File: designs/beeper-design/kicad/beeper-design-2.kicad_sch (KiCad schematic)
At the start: 26 parts, among them U14 EVPBB4A9B000, U15 EVPBB4A9B000, U16 EVPBB4A9B000, U4 DA7212-01UM2, U9 LSM6DSOXTR

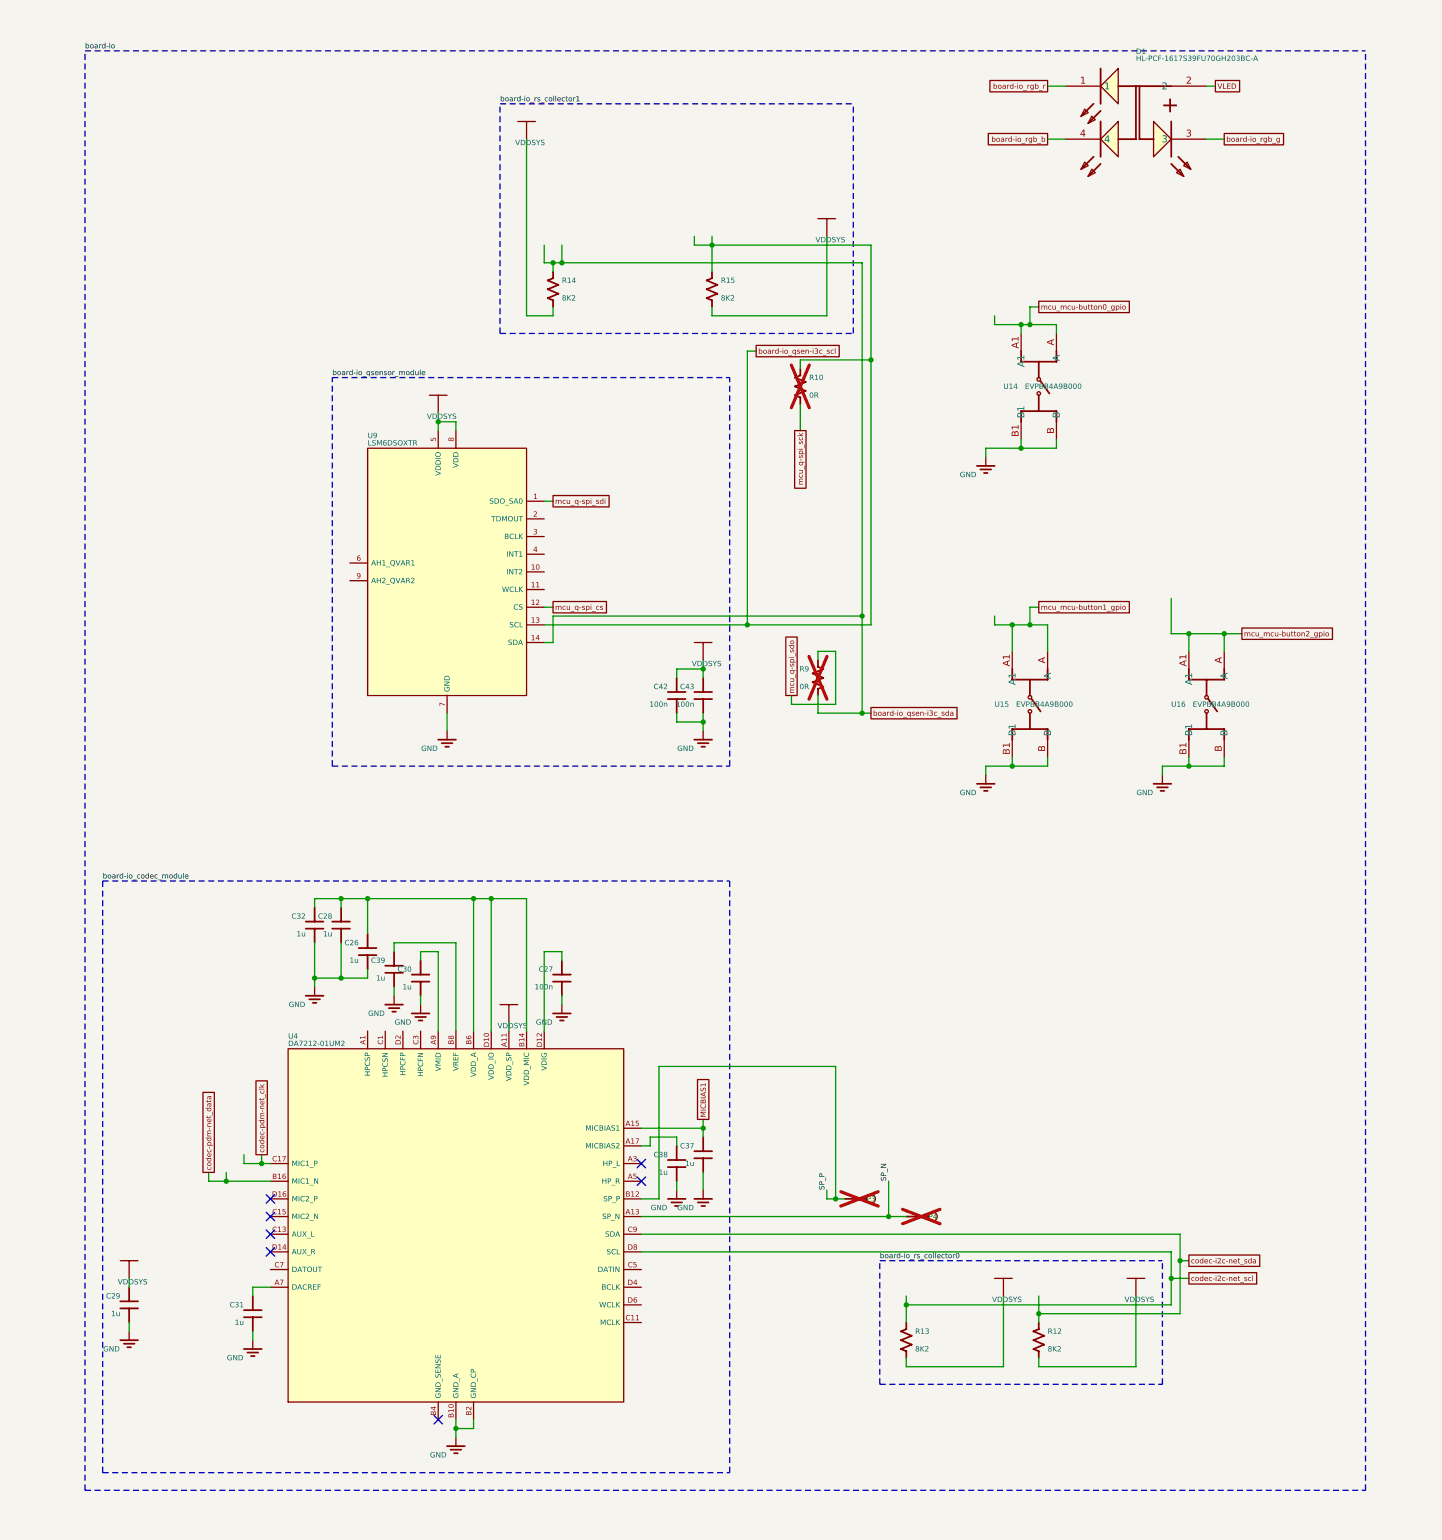
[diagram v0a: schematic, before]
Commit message: kicad exported data
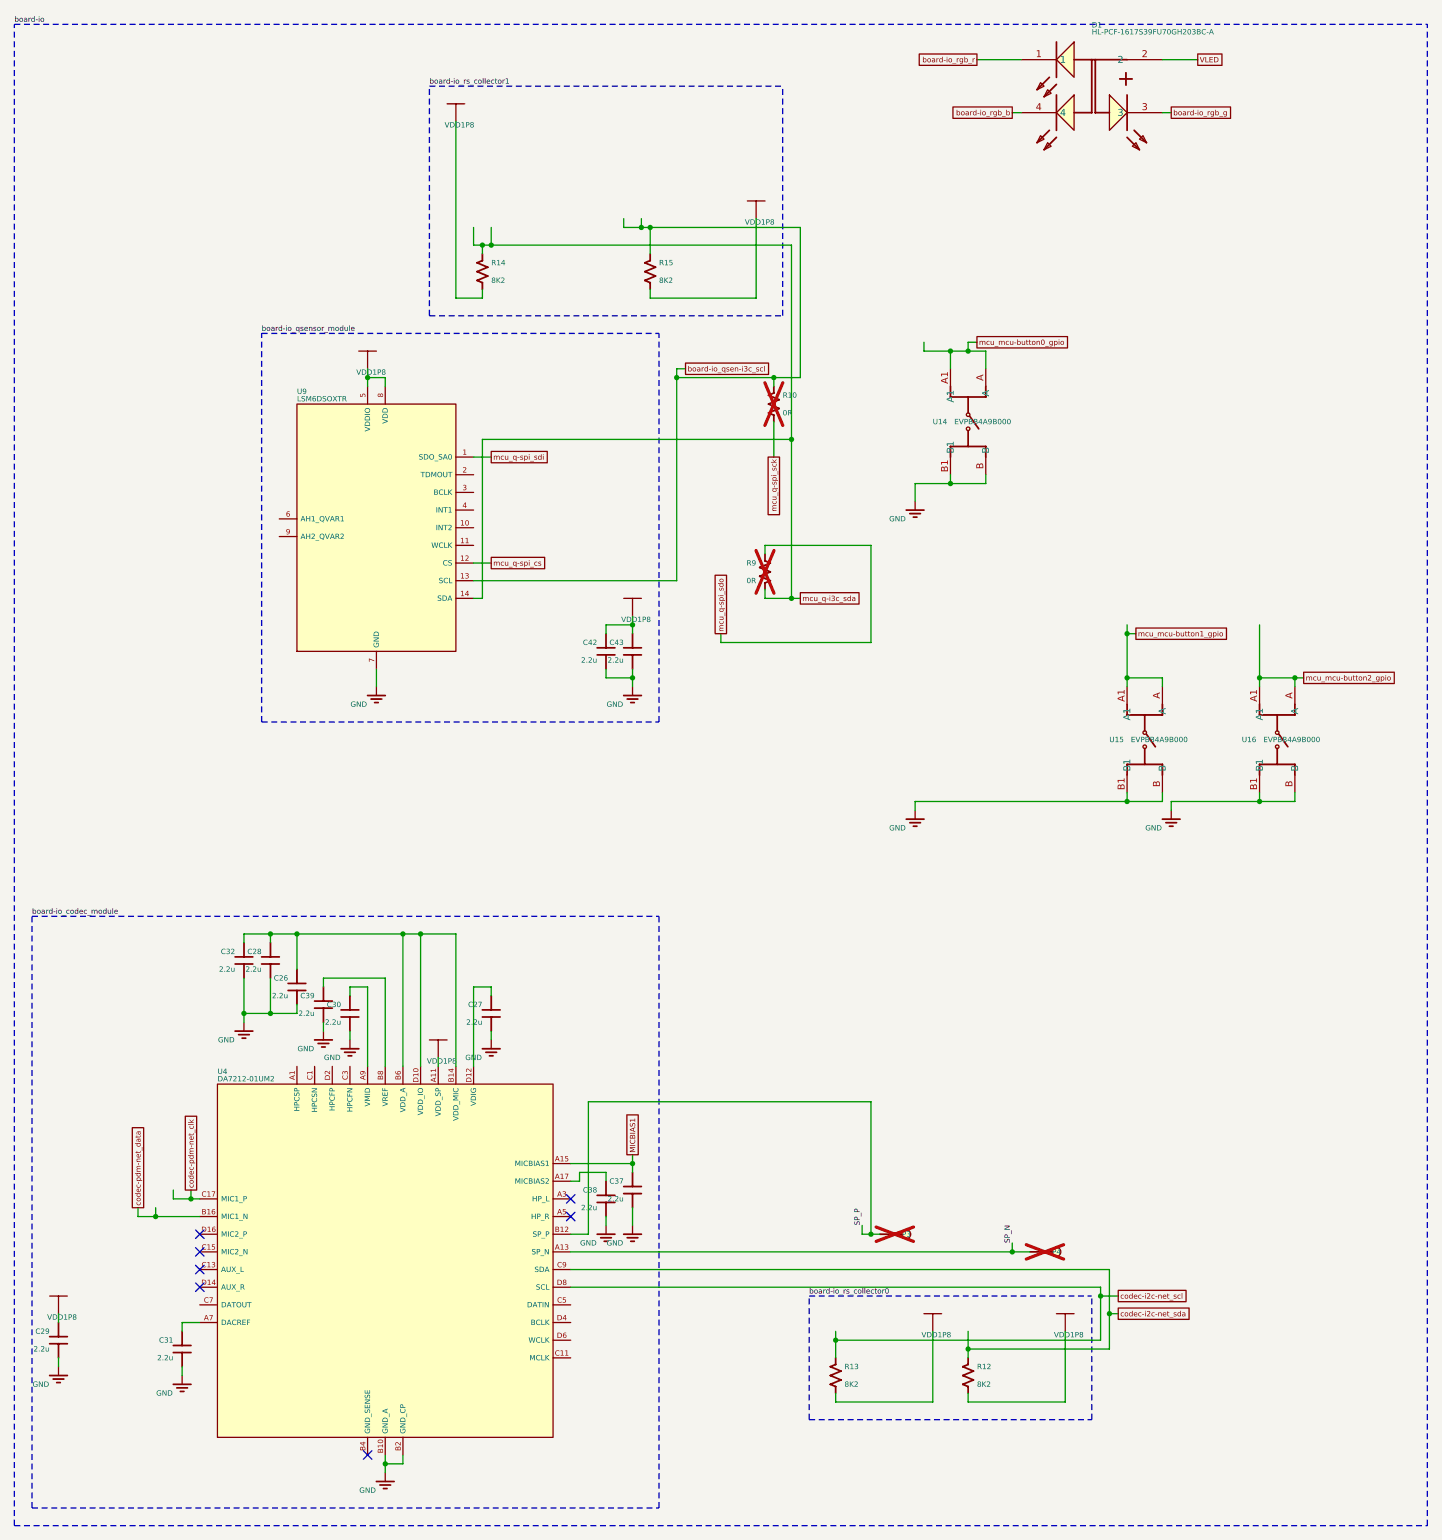
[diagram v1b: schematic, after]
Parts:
- removed C26: 1u, beeper-design:Pkg0201_27, symbol C76935_8
- removed C27: 100n, beeper-design:Pkg0201_38, symbol my_capacitor_13
- removed C28: 1u, beeper-design:Pkg0201_5, symbol C76935_1
- removed C29: 1u, beeper-design:Pkg0201_15, symbol C76935_5
- removed C30: 1u, beeper-design:Pkg0201_3, symbol C76935
- removed C31: 1u, beeper-design:Pkg0201_13, symbol C76935_4
- removed C32: 1u, beeper-design:Pkg0201_23, symbol C76935_6
- removed C37: 1u, beeper-design:Pkg0201_26, symbol C76935_7
- removed C38: 1u, beeper-design:Pkg0201_37, symbol C76935_10
- removed C39: 1u, beeper-design:Pkg0201_35, symbol C76935_9
- removed C42: 100n, beeper-design:Pkg0201_29, symbol my_capacitor_8
- removed C43: 100n, beeper-design:Pkg0201_39, symbol my_capacitor_14
- removed R10: 0R, beeper-design:Pkg0201_28, symbol my_resistor_8
- removed R12, R13: 8K2, beeper-design:Pkg0201_17, symbol my_resistor_4
- removed R14, R15: 8K2, beeper-design:Pkg0201_1, symbol my_resistor
- removed R9: 0R, beeper-design:Pkg0201_19, symbol my_resistor_5
- removed U4: DA7212-01UM2, beeper-design:LP_3, symbol component_1
- added C26: 2.2u, beeper-design:Pkg0201_19, symbol C335106_10
- added C27: 2.2u, beeper-design:Pkg0201_33, symbol C335106_21
- added C28: 2.2u, beeper-design:Pkg0201_46, symbol C335106_28
- added C29: 2.2u, beeper-design:Pkg0201_3, symbol C335106
- added C30: 2.2u, beeper-design:Pkg0201_43, symbol C335106_27
- added C31: 2.2u, beeper-design:Pkg0201, symbol C335106_36
- added C32: 2.2u, beeper-design:Pkg0201_12, symbol C335106_6
- added C37: 2.2u, beeper-design:Pkg0201_17, symbol C335106_8
- added C38: 2.2u, beeper-design:Pkg0201_31, symbol C335106_20
- added C39: 2.2u, beeper-design:Pkg0201_28, symbol C335106_18
- added C42: 2.2u, beeper-design:Pkg0201_21, symbol C335106_11
- added C43: 2.2u, beeper-design:Pkg0201_34, symbol C335106_22
- added R10: 0R, beeper-design:Pkg0201_20, symbol my_resistor_5
- added R12, R13: 8K2, beeper-design:Pkg0201_5, symbol my_resistor_1
- added R14, R15: 8K2, beeper-design:Pkg0201_42, symbol my_resistor_10
- added R9: 0R, beeper-design:Pkg0201_7, symbol my_resistor_2
- added U4: DA7212-01UM2, beeper-design:LP_3, symbol component
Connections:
- net GND: now also C26.1, C27.1, C28.1, C29.1, C30.1, C31.1, C32.1, C37.1, C38.1, C39.1, C42.1, C43.1, U4.B10 (GND_A), U4.B2 (GND_CP)
- net MICBIAS1: now also C37.2, U4.A15 (MICBIAS1)
- net SP_N: now also U4.A13 (SP_N)
- net SP_P: now also U4.B12 (SP_P)
- net board-io_qsen-i3c_scl: now also R10.1, R15.1
- net codec-i2c-net_scl: now also R13.1, U4.D8 (SCL)
- net codec-i2c-net_sda: now also R12.1, U4.C9 (SDA)
- net codec-pdm-net_clk: now also U4.C17 (MIC1_P)
- net codec-pdm-net_data: now also U4.B16 (MIC1_N)
- net mcu_q-spi_sck: now also R10.2
- net mcu_q-spi_sdo: now also R9.2
- net VDDSYS renamed VDD1P8
- net VDD1P8: now also C29.2, C42.2, C43.2, R12.2, R13.2, R14.2, R15.2, U4.A11 (VDD_SP)
- net board-io_qsen-i3c_sda renamed mcu_q-i3c_sda
- net mcu_q-i3c_sda: now also R14.1, R9.1
- new net: C39.2, U4.B8 (VREF)
- new net: C26.2, C28.2, C32.2, U4.B14 (VDD_MIC), U4.B6 (VDD_A), U4.D10 (VDD_IO)
- new net: C27.2, U4.D12 (VDIG)
- new net: C38.2, U4.A17 (MICBIAS2)
- new net: C31.2, U4.A7 (DACREF)
- new net: C30.2, U4.A9 (VMID)
